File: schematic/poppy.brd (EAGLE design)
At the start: 31 x 51.9 mm, 18 parts, among them Q1 8MHz, U1 ATMEGA16U4TQFP44, U2 MBI5030GFSOP-24

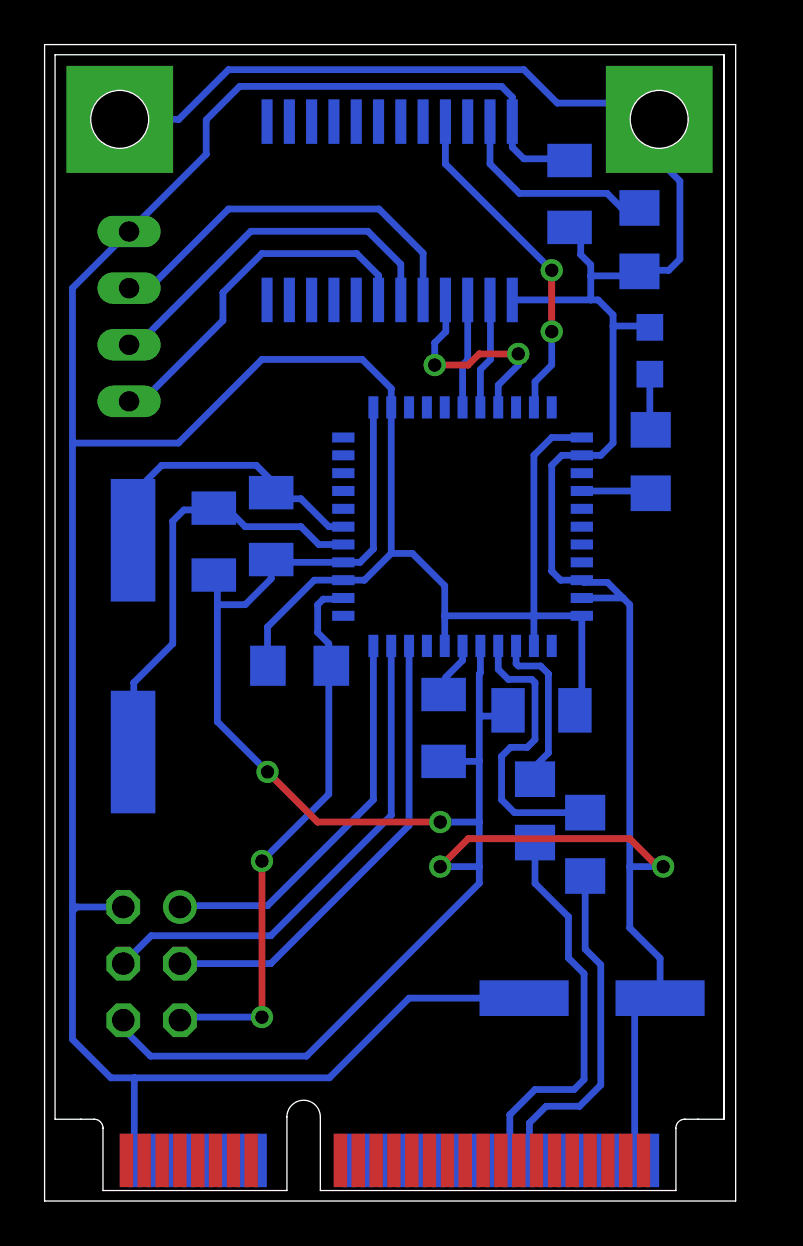
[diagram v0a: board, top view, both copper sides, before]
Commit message: first production
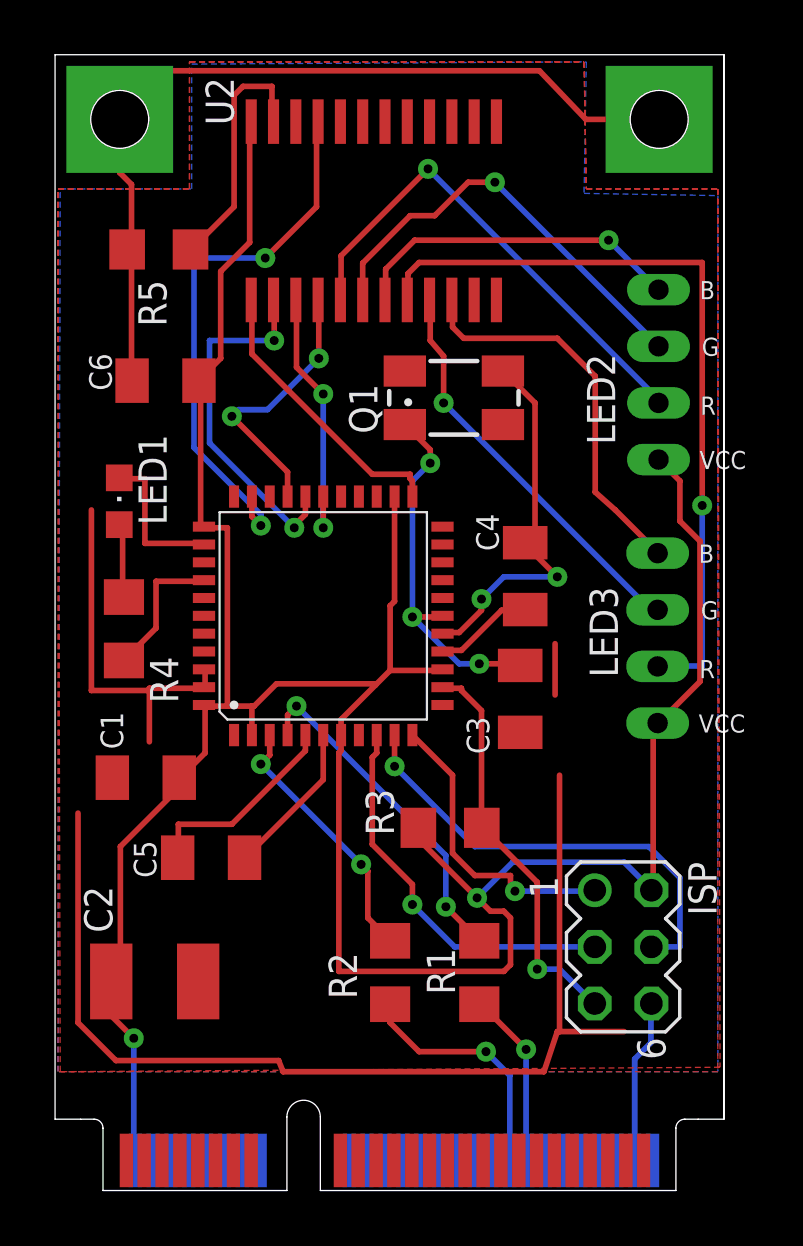
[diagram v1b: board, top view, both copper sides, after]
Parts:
- added LED3: CON-RGB-LED-EXT, _led-rgb:CON-RGB-LED-TH-EXT
- C2: device resistor:153CLV-0807 -> resistor:C1812
- Q1: device crystal:CSM-7X-DU -> crystal:CTS406
- moved R4 24.8 mm to (3.06, 25.2), flipped to the top
- moved LED1 24.7 mm to (2.85, 30.9), flipped to the top
- moved LED2 23.9 mm to (27.0, 36.6), flipped to the top, turned to 180 degrees
- moved R5 21.6 mm to (4.62, 42.2), flipped to the top, turned to 0 degrees
- moved ISP 21.2 mm to (25.4, 10.9), flipped to the top
- moved C6 20.0 mm to (4.92, 36.3), flipped to the top, turned to 180 degrees
- moved C2 19.6 mm to (4.44, 9.35), flipped to the top
- moved Q1 18.2 mm to (17.9, 35.5), flipped to the top, turned to 0 degrees
- moved C1 18.0 mm to (4.04, 18.5), flipped to the top, turned to 180 degrees
- moved C4 14.1 mm to (21.1, 27.5), flipped to the top
- moved C3 13.6 mm to (20.8, 22.0), flipped to the top
- moved C5 11.9 mm to (6.97, 14.9), flipped to the top, turned to 180 degrees
- moved R3 9.92 mm to (17.7, 16.2), flipped to the top, turned to 180 degrees
- moved R2 9.74 mm to (15.0, 9.75), flipped to the top
- moved R1 7.46 mm to (19.0, 9.75), flipped to the top
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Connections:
- new net N$11: LED3.3.R, U2.8
- new net N$12: LED3.2.G, U2.9
- new net N$13: LED3.1.B, U2.10
- net GND: now also C2.2; no longer C2.-
- net VCC: now also C2.1, LED3.4.VCC; no longer C2.+
- net XTAL2: now also Q1.3; no longer Q1.2
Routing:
- net N$11: track 0.00 -> 34.7 mm, vias 0 -> 1
- net GND: track 178.6 -> 146.5 mm, vias 4 -> 0
- net VCC: track 150.9 -> 131.5 mm, vias 0 -> 2
- net N$12: track 0.00 -> 18.3 mm, vias 0 -> 1
- net N$13: track 0.00 -> 17.7 mm
- net SDI: track 5.01 -> 16.3 mm, vias 0 -> 2
- net CLK0: track 15.1 -> 25.0 mm
- net D+: track 15.3 -> 7.95 mm, vias 0 -> 1
- net D-: track 18.3 -> 11.0 mm, vias 0 -> 1
- net DCLK: track 4.92 -> 12.1 mm, vias 0 -> 2
- net RESET: track 24.9 -> 18.1 mm, vias 2 -> 1
- net N$3: track 17.6 -> 22.4 mm, vias 0 -> 1
- net N$4: track 2.53 -> 6.98 mm
- net N$10: track 7.41 -> 11.8 mm, vias 0 -> 2
- net MISO: track 17.6 -> 13.4 mm, vias 0 -> 1
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- added copper zone on layer 1, net GND
- added copper zone on layer 16, net GND
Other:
- board size 31 x 51.9 mm -> 30 x 51 mm
